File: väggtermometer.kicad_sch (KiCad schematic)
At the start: 145 parts, among them J1 USB_C_Receptacle_USB2.0, J2 Conn_01x08, J4 NC, J8 Conn_01x02, Q1 BSS84, SW1 SW_MEC_5G, SW3 SW_MEC_5G, U1 ESP32-C3, U2 RT9080, U3 TC1047AxNB, U4 MCP73831, Y1 Crystal

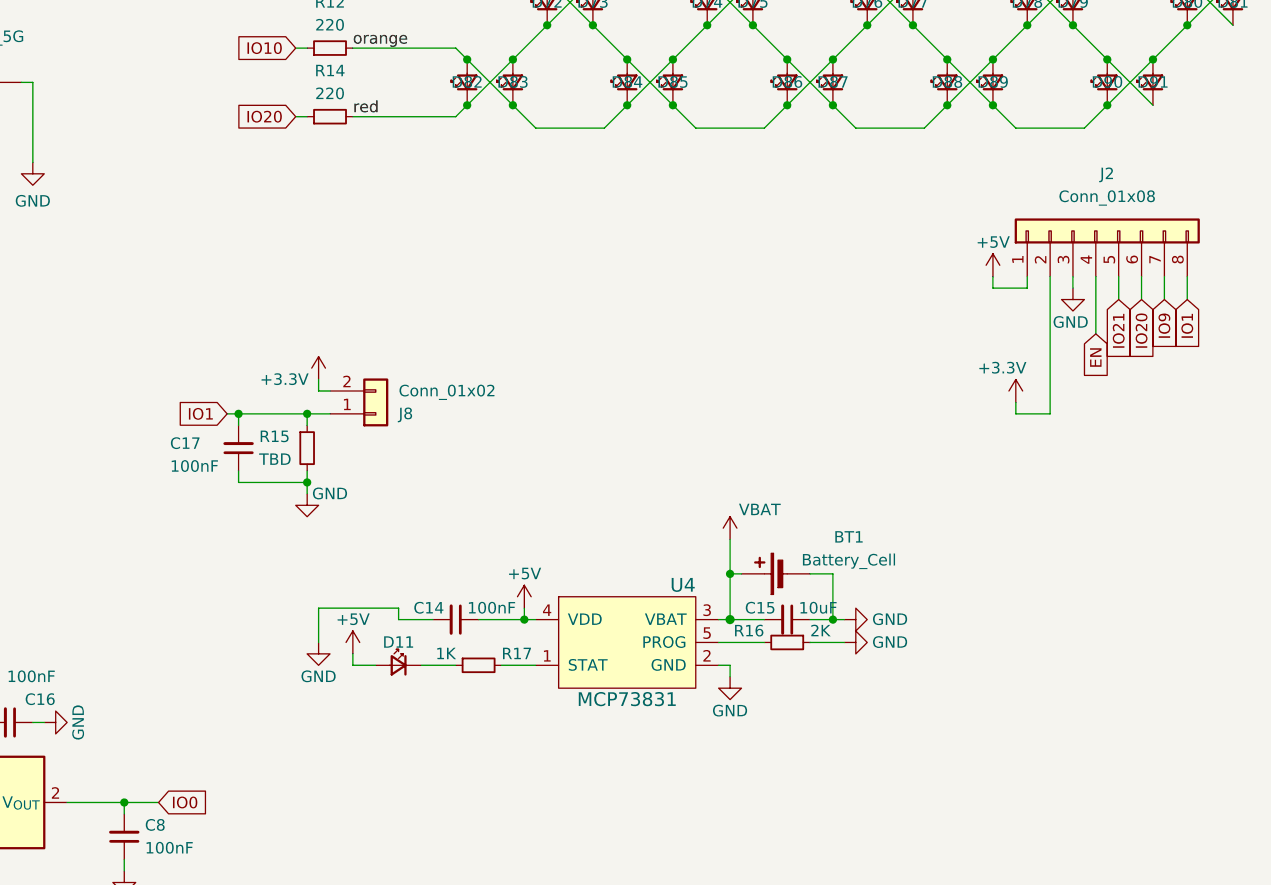
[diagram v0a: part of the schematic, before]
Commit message: info and stuff
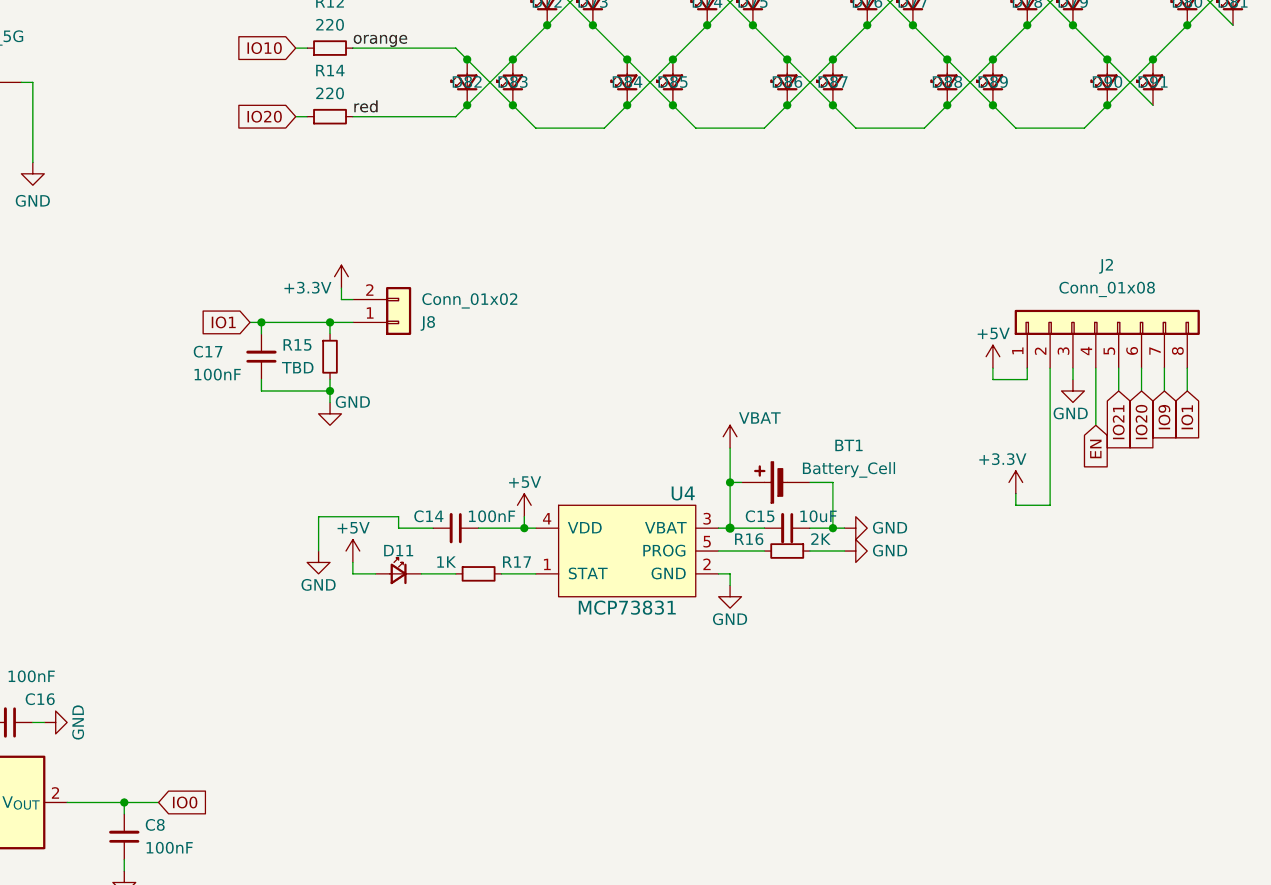
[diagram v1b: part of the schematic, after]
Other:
- moved on the sheet: BT1, C14, C15, C17, D11, J2, J8, R15, R16, R17, U4
